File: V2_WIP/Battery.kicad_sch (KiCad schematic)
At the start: 21 parts, among them J601 BATT, SW602 MSN22AFW01, U601 *IP5306, U602 STC3100IST

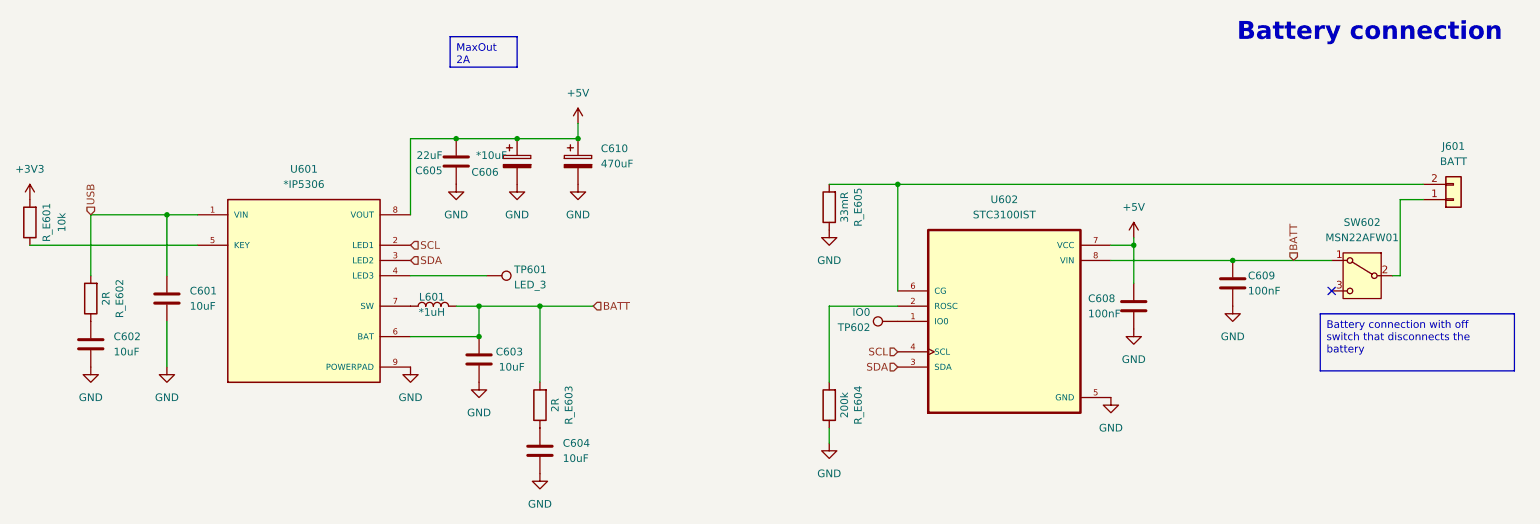
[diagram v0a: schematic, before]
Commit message: up to date i dont remember what changed
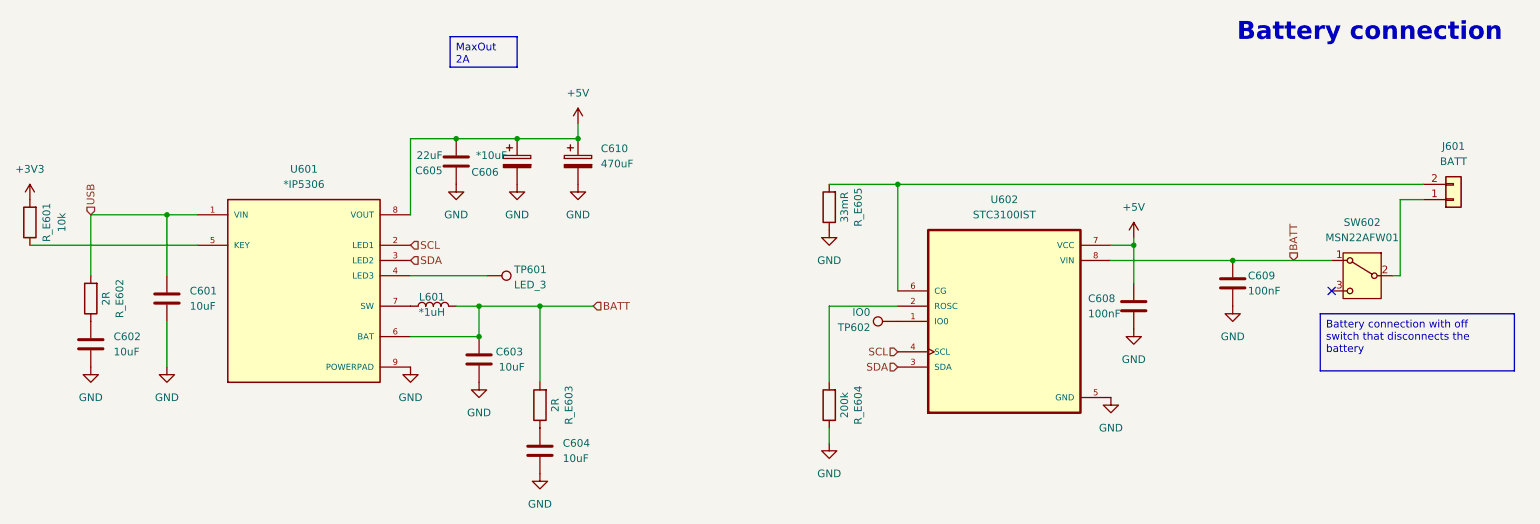
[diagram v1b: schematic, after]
